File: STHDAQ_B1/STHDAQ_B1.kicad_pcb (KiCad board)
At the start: 2 copper layers, 36 x 56 mm, 35 parts, among them J1 532611071, P1 S2B-PH-SM4-TB, P2 S2B-PH-SM4-TB, SW1 SW_Push, U1 IP5306, U2 102010448

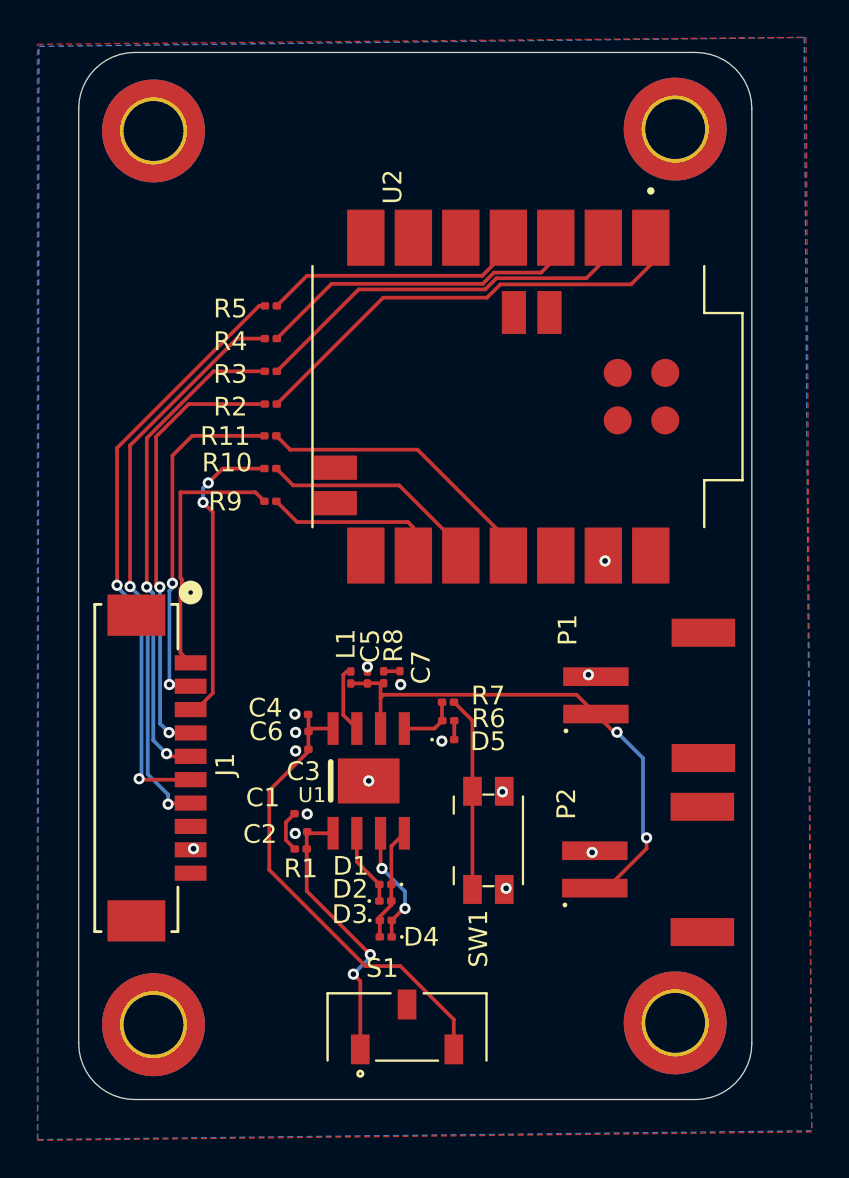
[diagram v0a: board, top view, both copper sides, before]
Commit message: B1 New
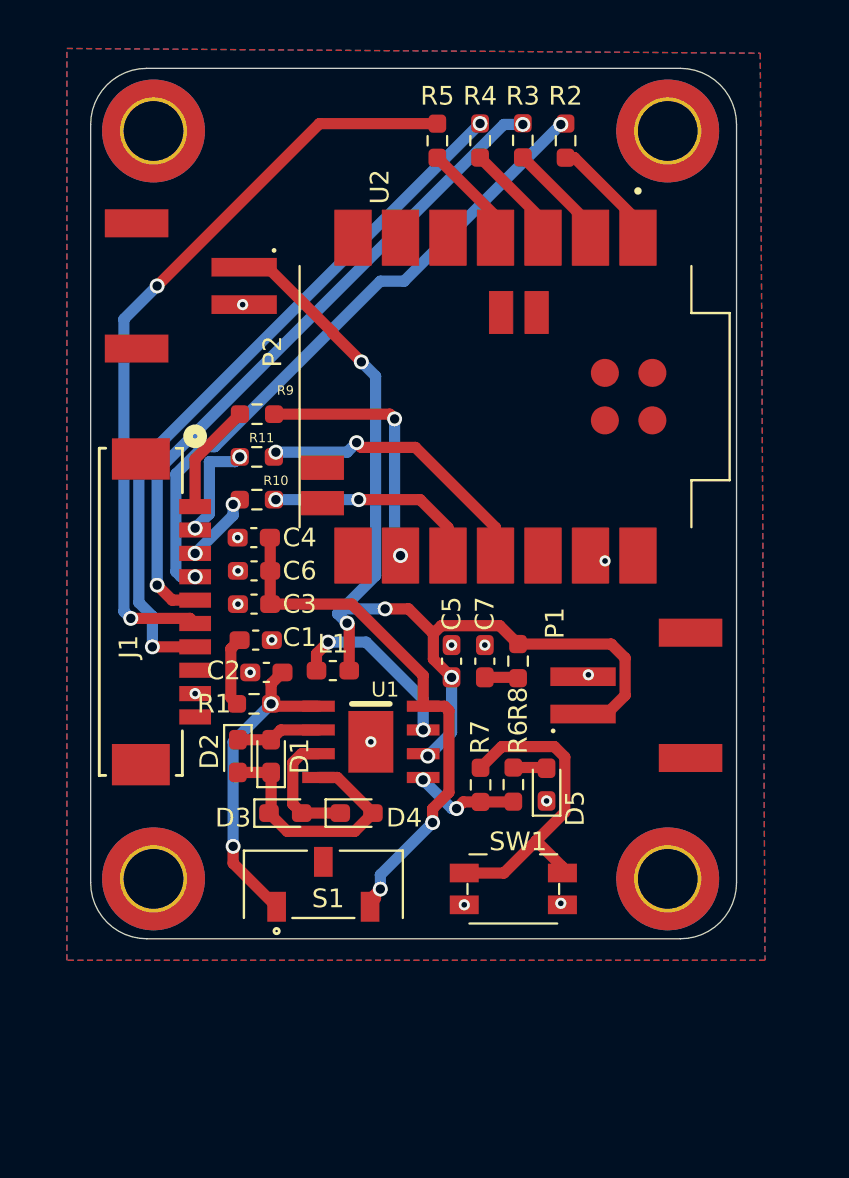
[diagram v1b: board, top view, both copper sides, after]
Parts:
- C1, C2, C3, C4, C5, C6, C7: footprint Capacitor_SMD:C_0201_0603Metric -> Capacitor_SMD:C_0603_1608Metric_Pad1.08x0.95mm_HandSolder
- D1, D2, D3, D4, D5: footprint LED_SMD:LED_0201_0603Metric -> LED_SMD:LED_0603_1608Metric_Pad1.05x0.95mm_HandSolder
- L1: footprint Inductor_SMD:L_0201_0603Metric -> Inductor_SMD:L_0603_1608Metric_Pad1.05x0.95mm_HandSolder
- R1, R10, R11, R2, R3, R4, R5, R6, R7, R8, R9: footprint Resistor_SMD:R_0201_0603Metric -> Resistor_SMD:R_0603_1608Metric_Pad0.98x0.95mm_HandSolder
- moved P2 36.4 mm to (145.9, 63.0), turned to 90 degrees
- moved R2 21.1 mm to (163.1, 55.2), turned to -90 degrees
- moved R3 18.3 mm to (160.8, 55.2), turned to -90 degrees
- moved R4 15.4 mm to (158.5, 55.2), turned to -90 degrees
- moved R5 12.5 mm to (156.2, 55.2), turned to -90 degrees
- moved D2 11.1 mm to (145.5, 88.1), turned to -90 degrees
- moved C4 9.80 mm to (146.4, 76.5)
- moved C1 9.59 mm to (146.5, 81.9)
- moved D1 9.19 mm to (147.3, 88.1), turned to 90 degrees
- moved C6 8.97 mm to (146.4, 78.2)
- moved S1 8.84 mm to (150.1, 95.0)
- moved C2 8.73 mm to (147.1, 83.7)
- moved J1 8.36 mm to (140.4, 80.4)
- moved C3 8.18 mm to (146.4, 80.0)
- moved R1 8.15 mm to (146.4, 85.3)
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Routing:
- net BAT: track 28.3 -> 55.7 mm, vias 2 -> 5
- net Net-(U2-A0/D0): track 24.5 -> 6.16 mm
- net Net-(U2-A1/D1): track 21.2 -> 5.79 mm
- net /DIN: track 18.8 -> 5.70 mm
- net /DOUT: track 16.4 -> 3.92 mm
- net Net-(U2-A2/D2): track 17.8 -> 5.68 mm
- net /DRDY: track 23.9 -> 35.0 mm
- net /CS: track 26.5 -> 35.7 mm
- net Net-(U2-A3/D3): track 14.3 -> 5.56 mm
- net /RESET: track 32.1 -> 40.8 mm
- net /SCLK: track 14.1 -> 5.94 mm
- net Net-(D1-K): track 6.09 -> 14.1 mm
- net /SYNC/PDWN: track 30.8 -> 38.1 mm
- net Net-(R7-Pad2): track 10.4 -> 17.2 mm
- net Net-(U1-SW): track 3.64 -> 9.78 mm, vias 0 -> 2
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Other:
- board size 36 x 56 mm -> 34.5 x 46.6 mm
